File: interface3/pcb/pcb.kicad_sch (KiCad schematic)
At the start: 56 parts, among them J1 PORT1, J2 PORT2, J3 PORT3/4, J4 POWER, SW1 Pico Run, T1 78602/8JC, T2 78602/8JC, U1 DS34LV86T, U2 DS34LV87T, U3 Pico_W

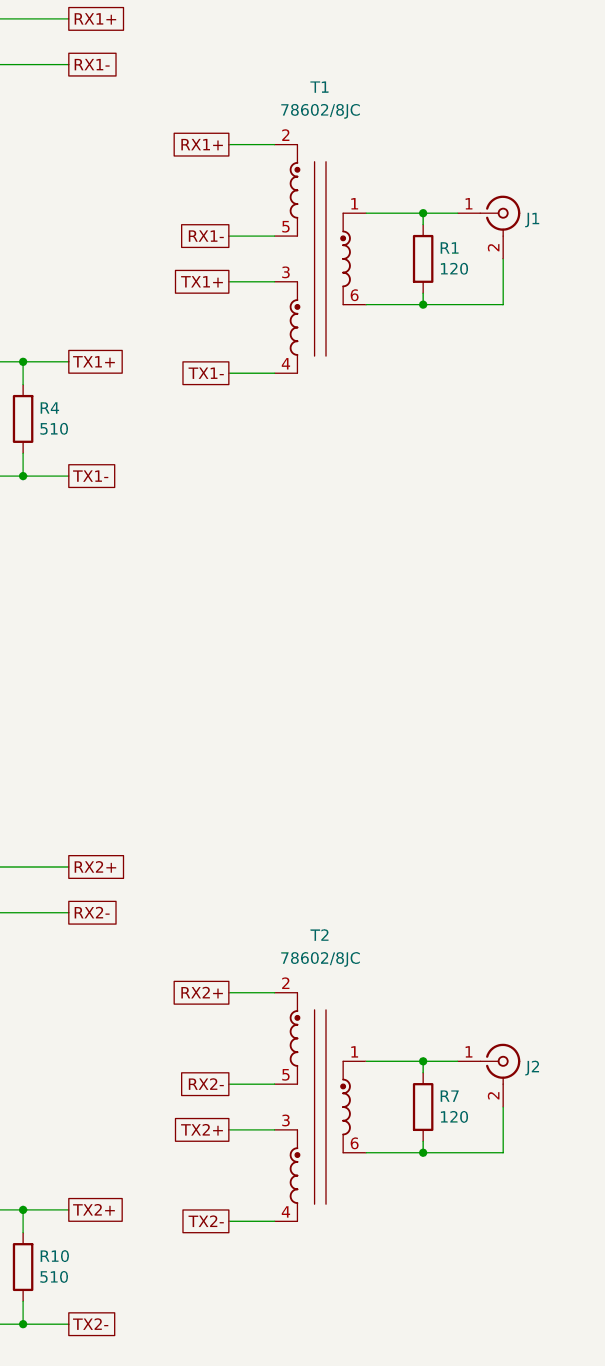
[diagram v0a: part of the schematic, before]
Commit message: finish layout (again) - this version has not been produced yet
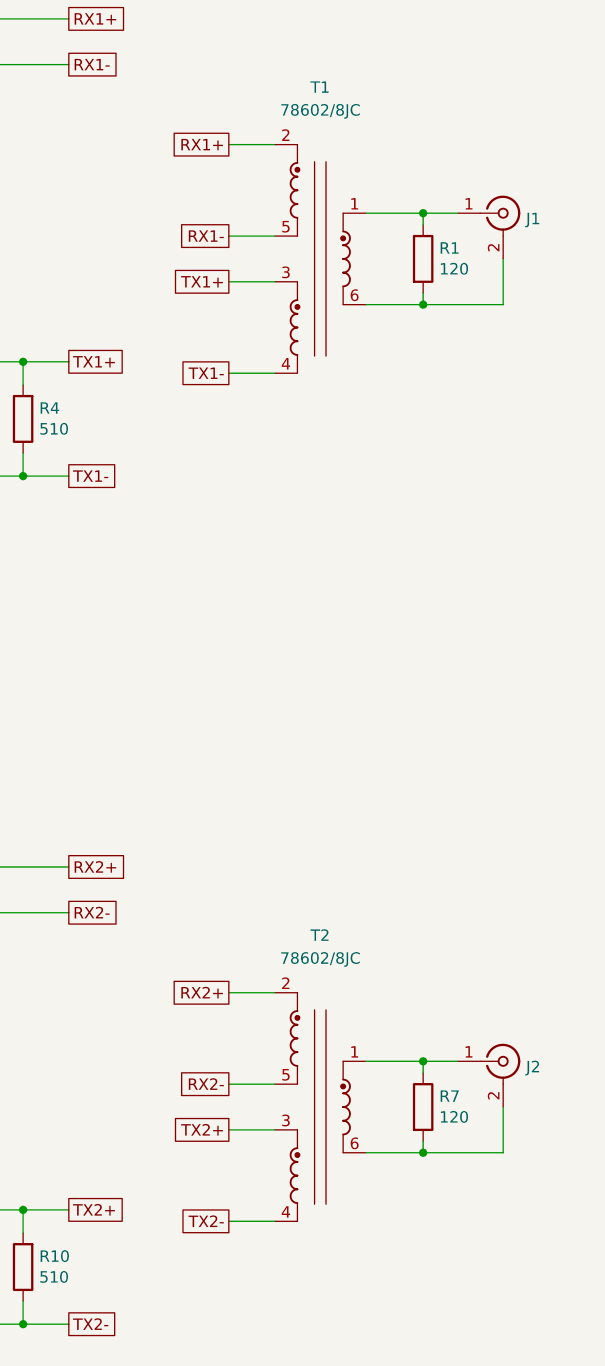
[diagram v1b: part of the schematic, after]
